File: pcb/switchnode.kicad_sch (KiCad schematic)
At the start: 4 parts, among them Q1 BC817, Q2 IRLML6402

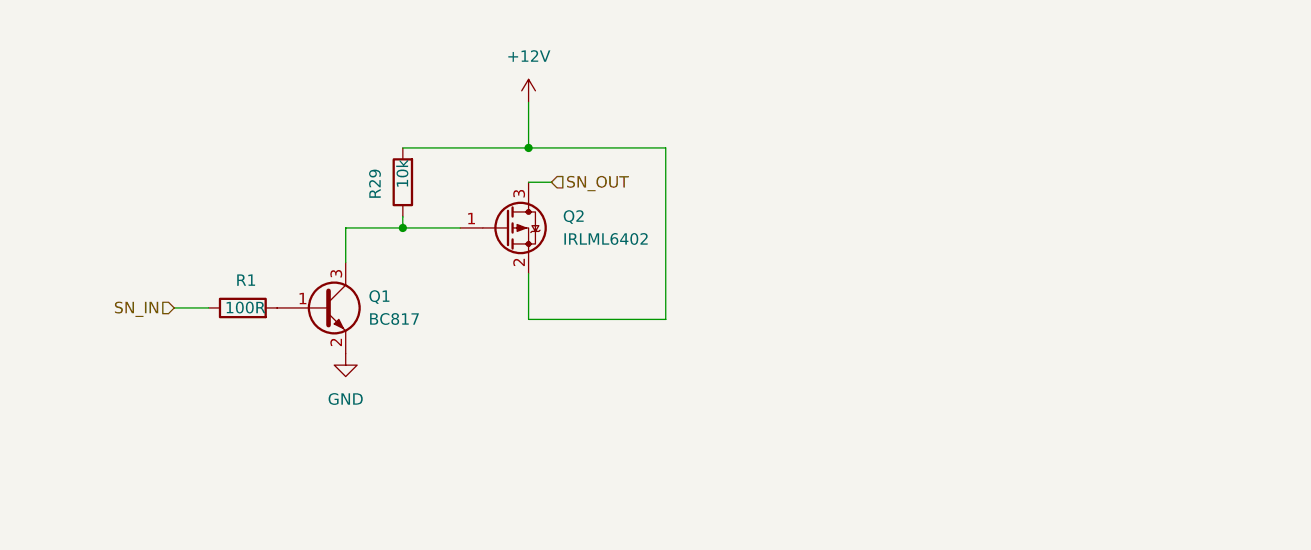
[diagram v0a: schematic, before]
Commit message: recovered lost pcb
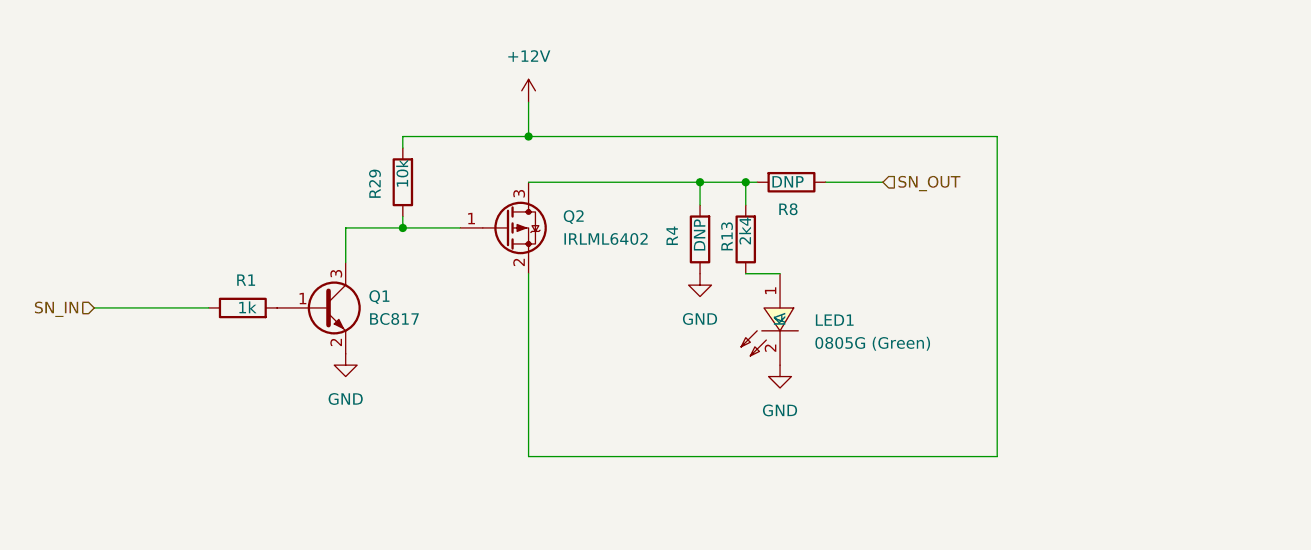
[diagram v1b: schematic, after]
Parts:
- added LED1: 0805G (Green), lcsc:LED0805-R-RD, symbol lcsc:0805G(Green)
- added R13: 2k4, Resistor_SMD:R_0603_1608Metric, symbol Device:R
- added R4, R8: DNP, Resistor_THT:R_Axial_DIN0207_L6.3mm_D2.5mm_P7.62mm_Horizontal, symbol Device:R
- R1: value 100R -> 1k
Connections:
- net GND: now also LED1.2 (K), R4.1
- net SN_OUT: now also R8.1; no longer Q2.3 (D)
- new net: LED1.1 (A), R13.1
- new net: Q2.3 (D), R13.2, R4.2, R8.2

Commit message: fixed the dumb schematic
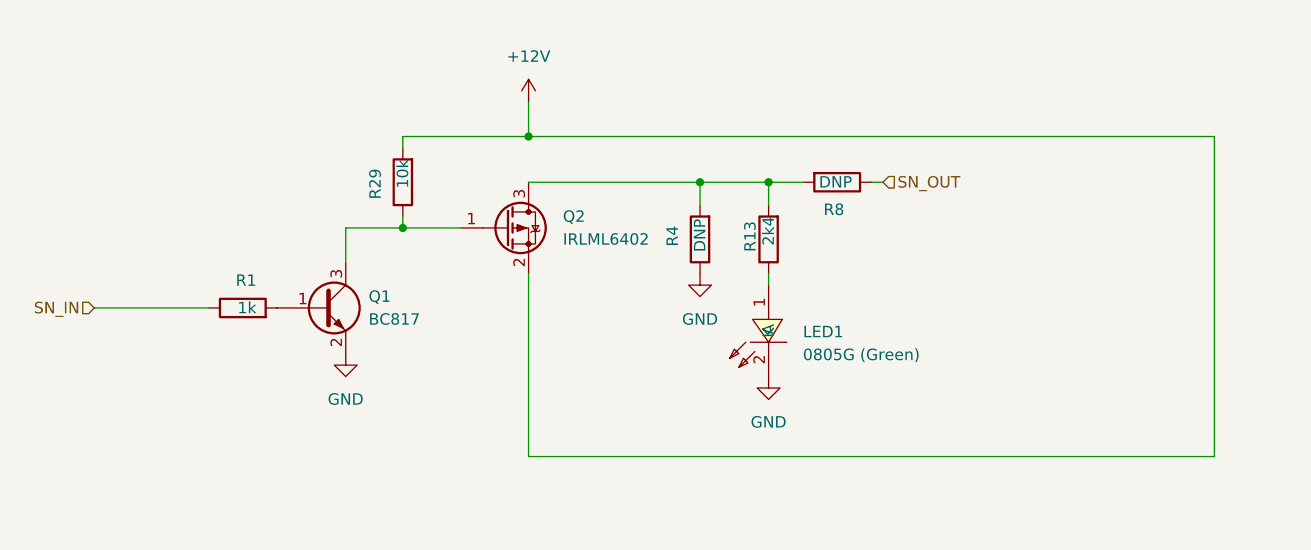
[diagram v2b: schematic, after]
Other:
- moved on the sheet: LED1, R13, R8
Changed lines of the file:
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@@
 	(paper "A4")
+	(junction
+		(at 173.99 83.82)
+		(diameter 0)
+		(color 0 0 0 0)
+	)
 	(junction
 		(at 133.35 88.9)
@@
 	)
 	(junction
-		(at 171.45 83.82)
-		(diameter 0)
-		(color 0 0 0 0)
-	)
-	(junction
 		(at 166.37 83.82)
 		(diameter 0)
@@
 	(wire
 		(pts
-			(xy 175.26 93.98) (xy 171.45 93.98)
+			(xy 173.99 95.25) (xy 173.99 93.98)
 		)
 		(stroke
@@
 	(wire
 		(pts
-			(xy 199.39 78.74) (xy 147.32 78.74)
-		)
-		(stroke
-			(width 0)
-			(type default)
-		)
-	)
-	(wire
-		(pts
-			(xy 147.32 114.3) (xy 199.39 114.3)
-		)
-		(stroke
-			(width 0)
-			(type default)
-		)
-	)
-	(wire
-		(pts
-			(xy 180.34 83.82) (xy 186.69 83.82)
+			(xy 223.52 78.74) (xy 147.32 78.74)
+		)
+		(stroke
+			(width 0)
+			(type default)
+		)
+	)
+	(wire
+		(pts
+			(xy 147.32 114.3) (xy 223.52 114.3)
+		)
+		(stroke
+			(width 0)
+			(type default)
+		)
+	)
+	(wire
+		(pts
+			(xy 185.42 83.82) (xy 186.69 83.82)
 		)
 		(stroke
@@
 	(wire
 		(pts
-			(xy 199.39 114.3) (xy 199.39 78.74)
+			(xy 223.52 114.3) (xy 223.52 78.74)
 		)
 		(stroke
@@
 	(wire
 		(pts
-			(xy 166.37 83.82) (xy 171.45 83.82)
+			(xy 173.99 83.82) (xy 177.8 83.82)
+		)
+		(stroke
+			(width 0)
+			(type default)
+		)
+	)
+	(wire
+		(pts
+			(xy 166.37 83.82) (xy 173.99 83.82)
 		)
 		(stroke
@@
 	(wire
 		(pts
-			(xy 171.45 86.36) (xy 171.45 83.82)
+			(xy 173.99 86.36) (xy 173.99 83.82)
 		)
 		(stroke
@@
 		(pts
 			(xy 133.35 87.63) (xy 133.35 88.9)
-		)
-		(stroke
-			(width 0)
-			(type default)
-		)
-	)
-	(wire
-		(pts
-			(xy 171.45 83.82) (xy 172.72 83.82)
 		)
 		(stroke
@@
 	(symbol
 		(lib_id "Device:R")
-		(at 171.45 90.17 180)
+		(at 173.99 90.17 180)
 		(unit 1)
 		(exclude_from_sim no)
@@
 		(dnp no)
 		(property "Reference" "R13"
-			(at 169.418 88.138 90)
+			(at 171.958 88.138 90)
 			(effects
 				(font
@@
 		)
 		(property "Value" "2k4"
-			(at 171.45 87.63 90)
+			(at 173.99 87.63 90)
 			(effects
 				(font
@@
 		)
 		(property "Footprint" "Resistor_SMD:R_0603_1608Metric"
-			(at 173.228 90.17 90)
+			(at 175.768 90.17 90)
 			(effects
 				(font
@@
 		)
 		(property "Datasheet" "~"
-			(at 171.45 90.17 0)
+			(at 173.99 90.17 0)
 			(effects
 				(font
@@
 		)
 		(property "Description" ""
-			(at 171.45 90.17 0)
+			(at 173.99 90.17 0)
 			(effects
 				(font
@@
 	(symbol
 		(lib_id "Device:R")
-		(at 176.53 83.82 270)
+		(at 181.61 83.82 270)
 		(unit 1)
 		(exclude_from_sim no)
@@
 		(dnp no)
 		(property "Reference" "R8"
-			(at 175.006 86.868 90)
+			(at 180.086 86.868 90)
 			(effects
 				(font
@@
 		)
 		(property "Value" "DNP"
-			(at 174.244 83.82 90)
+			(at 179.578 83.82 90)
 			(effects
 				(font
@@
 		)
 		(property "Footprint" "Resistor_THT:R_Axial_DIN0207_L6.3mm_D2.5mm_P7.62mm_Horizontal"
-			(at 176.53 82.042 90)
+			(at 181.61 82.042 90)
 			(effects
 				(font
@@
 		)
 		(property "Datasheet" "~"
-			(at 176.53 83.82 0)
+			(at 181.61 83.82 0)
 			(effects
 				(font
@@
 		)
 		(property "Description" ""
-			(at 176.53 83.82 0)
+			(at 181.61 83.82 0)
 			(effects
 				(font
@@
 		(lib_name "GND_1")
 		(lib_id "power:GND")
-		(at 175.26 104.14 0)
+		(at 173.99 105.41 0)
 		(unit 1)
 		(exclude_from_sim no)
@@
 		(fields_autoplaced yes)
 		(property "Reference" "#PWR015"
-			(at 175.26 110.49 0)
+			(at 173.99 111.76 0)
 			(effects
 				(font
@@
 		)
 		(property "Value" "GND"
-			(at 175.26 109.22 0)
+			(at 173.99 110.49 0)
 			(effects
 				(font
@@
 		)
 		(property "Footprint" ""
-			(at 175.26 104.14 0)
+			(at 173.99 105.41 0)
 			(effects
 				(font
@@
 		)
 		(property "Datasheet" ""
-			(at 175.26 104.14 0)
+			(at 173.99 105.41 0)
 			(effects
 				(font
@@
 		)
 		(property "Description" "Power symbol creates a global label with name \"GND\" , ground"
-			(at 175.26 104.14 0)
+			(at 173.99 105.41 0)
 			(effects
 				(font
@@
 	(symbol
 		(lib_id "lcsc:0805G(Green)")
-		(at 175.26 99.06 90)
+		(at 173.99 100.33 90)
 		(unit 1)
 		(exclude_from_sim no)
@@
 		(fields_autoplaced yes)
 		(property "Reference" "LED1"
-			(at 179.07 99.1849 90)
+			(at 177.8 100.4549 90)
 			(effects
 				(font
@@
 		)
 		(property "Value" "0805G (Green)"
-			(at 179.07 101.7249 90)
+			(at 177.8 102.9949 90)
 			(effects
 				(font
@@
 		)
 		(property "Footprint" "lcsc:LED0805-R-RD"
-			(at 182.88 99.06 0)
+			(at 181.61 100.33 0)
 			(effects
 				(font
@@
 		)
 		(property "Datasheet" "https://lcsc.com/product-detail/Light-Emitting-Diodes-LED_Green-0805-Highlighted_C2297.html"
-			(at 185.42 99.06 0)
+			(at 184.15 100.33 0)
 			(effects
 				(font
@@
 		)
 		(property "Description" ""
-			(at 175.26 99.06 0)
+			(at 173.99 100.33 0)
 			(effects
 				(font
@@
 		)
 		(property "LCSC Part" "C2297"
-			(at 187.96 99.06 0)
-			(effects
-				(font
+			(at 186.69 100.33 0)
+			(effects
+				(font

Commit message: learned from my mistakes
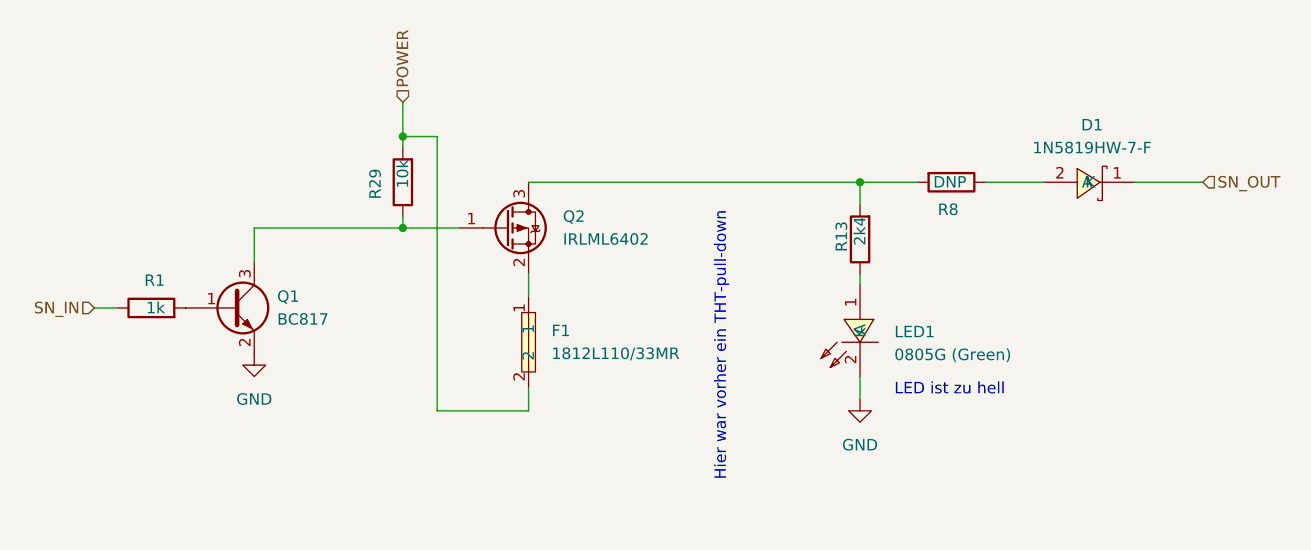
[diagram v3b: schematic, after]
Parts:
- removed R4: DNP, Resistor_THT:R_Axial_DIN0207_L6.3mm_D2.5mm_P7.62mm_Horizontal, symbol Device:R
- added D1: 1N5819HW-7-F, lcsc:SOD-123_L2.7-W1.6-LS3.7-RD, symbol lcsc:1N5819HW-7-F
- added F1: 1812L110/33MR, lcsc:F1812, symbol lcsc:1812L110_33MR
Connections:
- net SN_OUT: now also D1.1 (K); no longer R8.1
- net +12V: no longer names the net of Q2.2 (S)
- net +12V: now also F1.1; no longer R29.2
- new net: D1.2 (A), R8.1
- new net POWER: F1.2, R29.2
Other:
- note added: "Hier war vorher ein THT-pull-down"
- note added: "LED ist zu hell"
- moved on the sheet: LED1, Q1, R1, R13, R8
